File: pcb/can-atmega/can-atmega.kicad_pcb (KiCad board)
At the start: 2 copper layers, 36.6 x 46.5 mm, 31 parts, among them J1 Screw_Terminal_01x02, J2 Screw_Terminal_01x02, J3 Conn_01x04_Female, J4 Conn_01x02_Female, J5 Conn_01x08_Female, U1 LM1117-5.0, U2 TJA1051T, U3 MCP2515-xSO, U4 ATmega328P-A, X1 16MHz, X2 16MHz

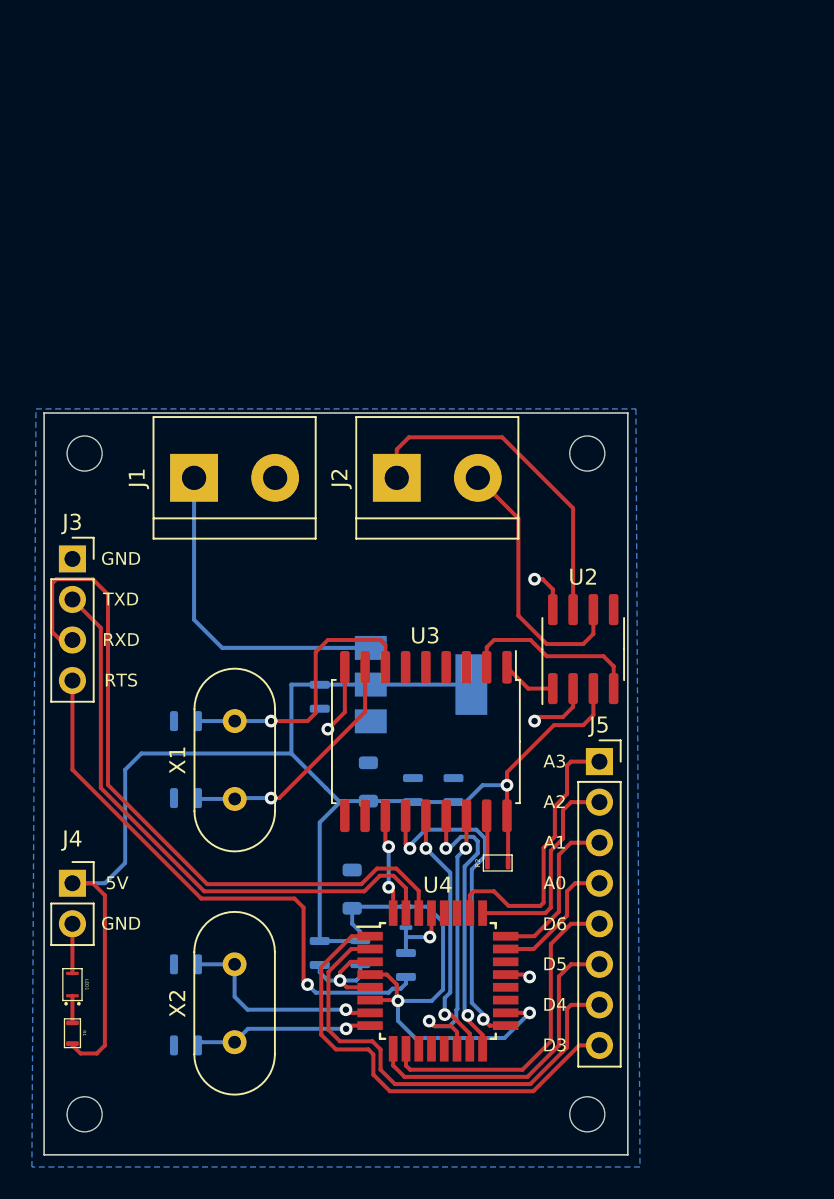
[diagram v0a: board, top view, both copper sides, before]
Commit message: motor module
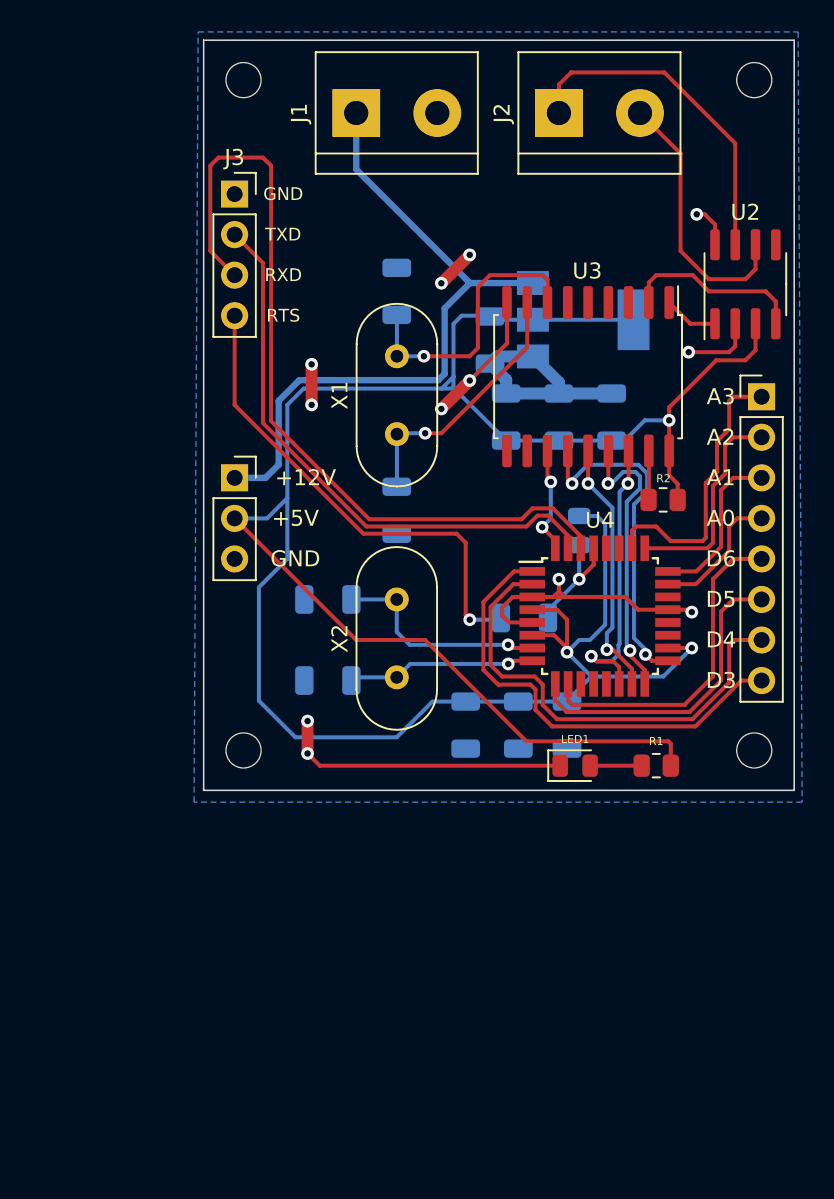
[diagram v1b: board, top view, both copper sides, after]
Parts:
- removed J5: Conn_01x08_Female, Connector_PinSocket_2.54mm:PinSocket_1x08_P2.54mm_Vertical
- C1, C10, C11, C12, C3, C4, C5, C6, C7, C9: footprint Capacitor_SMD_Custom:C_KEM_0805_2.0x1.25mm -> Capacitor_SMD:C_1206_3216Metric
- C2, C8: footprint Capacitor_SMD_Custom:C_TAJ_3516_Bauform_A -> Capacitor_SMD:C_1206_3216Metric
- J4: value Conn_01x02_Female -> Connector_female; footprint Connector_PinSocket_2.54mm:PinSocket_1x02_P2.54mm_Vertical -> CAN_ATmega:Connector_female
- LED1: footprint LED_SMD_Custom:LED_EL_0603_GR1_1608 -> LED_SMD:LED_0805_2012Metric
- R1, R2, R3: footprint Resistors_SMD_Custom:R_SPR-0603_1.6x0.8mm -> Resistor_SMD:R_0805_2012Metric
- moved R1 40.2 mm to (168.7, 114.6), turned to 180 degrees
- moved LED1 34.4 mm to (163.6, 114.6), turned to 0 degrees
- moved J4 34.2 mm to (157.5, 99.1)
- moved C6 30.0 mm to (152.4, 84.8), turned to -90 degrees
- moved R3 26.5 mm to (163.8, 99.8)
- moved REF** 25.6 mm to (174.8, 71.6)
- moved REF** 25.4 mm to (142.8, 71.6)
- moved C4 25.4 mm to (165.9, 92.7)
- moved C3 25.1 mm to (162.6, 92.7)
- moved REF** 25.1 mm to (174.8, 113.6)
- moved J1 25.0 mm to (149.9, 73.7)
- moved J2 25.0 mm to (162.6, 73.7)
- moved J3 25.0 mm to (142.2, 78.7)
- moved U1 25.0 mm to (164.1, 86.6)
- moved U2 25.0 mm to (174.2, 84.4)
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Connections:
- J1 pad 1: /12V -> +12V
- J4 pad 1: +5V -> +12V
- J4 pad 2: GND -> +5V
- U1 pad 3: /12V -> +12V
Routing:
- net GND: track 24.4 -> 70.4 mm, vias 5 -> 12
- net +5V: track 124.3 -> 167.7 mm
- net +12V: track 0.00 -> 42.1 mm
- net /12V: track 20.7 -> 0.00 mm
- net U4_RXD: track 44.9 -> 51.4 mm
- net U4_RTS: track 35.6 -> 30.6 mm
- net /U4_RESET: track 4.64 -> 7.69 mm
- net /LED1: track 1.70 -> 3.23 mm
- net /U3_OSC_1: track 15.6 -> 16.5 mm
- net U4_TXD: track 36.6 -> 35.9 mm
- net /U4_OSC_1: track 13.2 -> 13.8 mm
- net /U4_OSC_2: track 11.3 -> 11.8 mm
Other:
- board size 36.6 x 46.5 mm -> 37 x 47 mm
- board text removed: "5V"
- board text removed: "A0"
- board text removed: "A1"
- board text removed: "A2"
- board text removed: "A3"
- board text removed: "D3"
- board text removed: "D4"
- board text removed: "D5"
- board text removed: "D6"
